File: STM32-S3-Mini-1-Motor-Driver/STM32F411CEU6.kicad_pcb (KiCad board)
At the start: 2 copper layers, 77.3 x 60.5 mm, 47 parts, among them J1 USB_C_Receptacle_USB2.0, J10 5V, J11 3.3V, J12 4.5-36V, J2 MOTOR_1_OUT, J3 MOTOR_2_OUT, J4 MOTOR_3_OUT, J5 MOTOR_4_OUT, J6 Conn_01x15_Pin, J7 Conn_01x12_Pin, J8 Conn_01x02_Pin, Q2 AOD4185, SW2 EN, SW3 SLW-66527511-SMT-TR, U1 PCAL6408ABS, U2 ESP32-S3-MINI-1, U3 PRTR5V0U2X, U4 L293D, U5 TPS62160DSG, U6 L293D

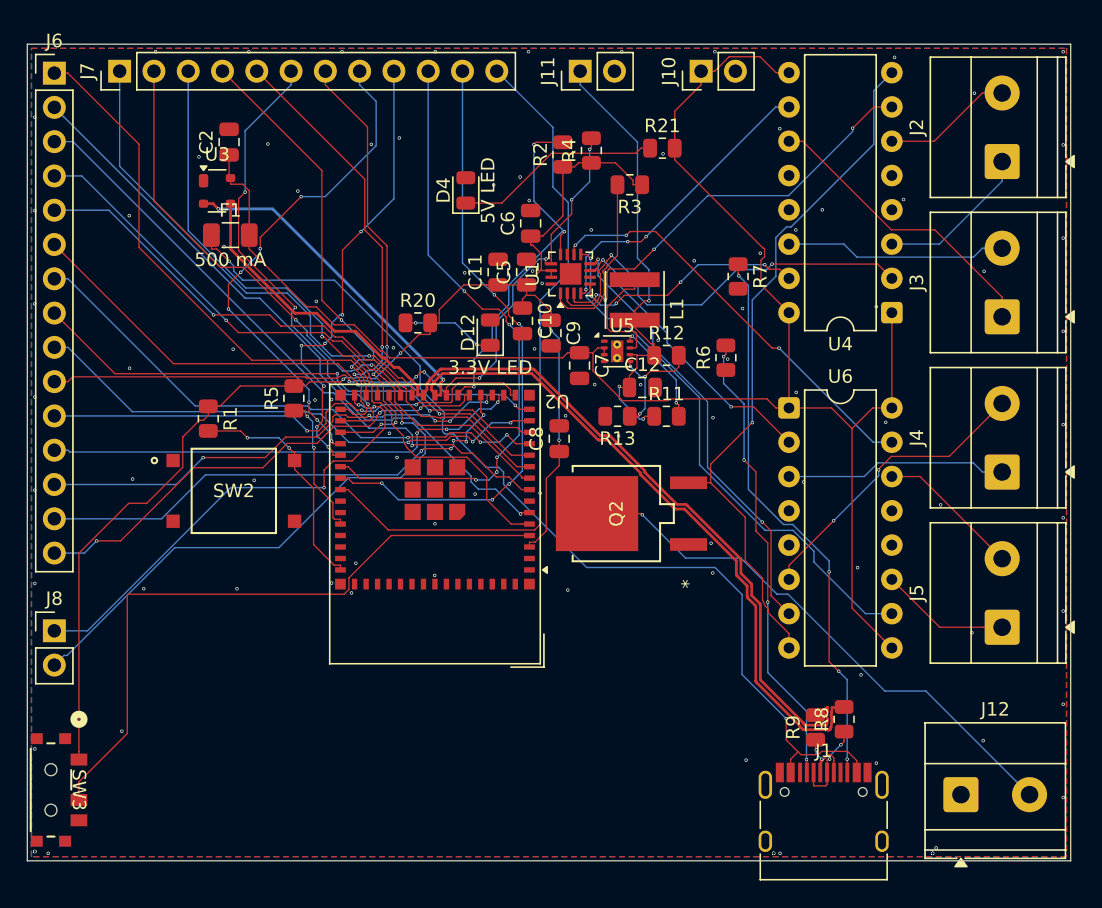
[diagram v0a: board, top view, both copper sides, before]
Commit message: You slongoid
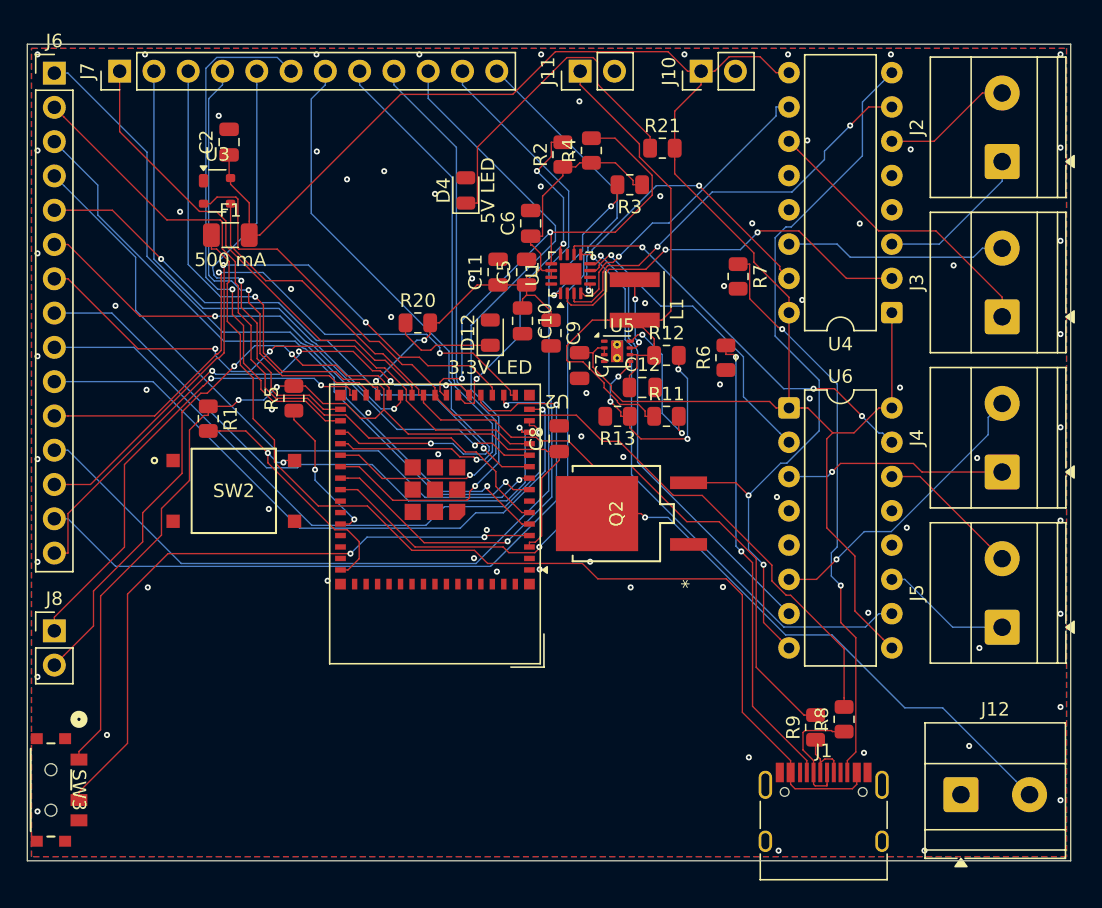
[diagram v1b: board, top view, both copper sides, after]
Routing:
- net Net-(J6-Pin_14): track 37.3 -> 54.4 mm, vias 5 -> 1
- net Net-(J6-Pin_12): track 36.0 -> 52.7 mm, vias 3 -> 1
- net +3.3V: track 34.0 -> 47.1 mm, vias 3 -> 0
- net Net-(J7-Pin_7): track 33.4 -> 45.8 mm, vias 4 -> 1
- net Net-(J6-Pin_13): track 36.3 -> 47.4 mm, vias 5 -> 2
- net Net-(J6-Pin_10): track 37.3 -> 48.2 mm, vias 4 -> 1
- net +5V: track 126.1 -> 136.8 mm
- net Net-(J7-Pin_9): track 34.3 -> 44.4 mm, vias 7 -> 1
- net Net-(D4-K): track 15.3 -> 24.8 mm
- net /I2C1_SDA: track 25.8 -> 34.7 mm, vias 4 -> 2
- net Net-(U5-FB): track 9.23 -> 17.6 mm, vias 3 -> 4
- net Net-(J6-Pin_9): track 39.1 -> 47.4 mm, vias 3 -> 1
- net Net-(J6-Pin_11): track 38.2 -> 46.4 mm, vias 3 -> 2
- net Net-(J7-Pin_11): track 46.6 -> 54.5 mm, vias 5 -> 1
- net Net-(J6-Pin_8): track 39.2 -> 46.6 mm, vias 2 -> 1
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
